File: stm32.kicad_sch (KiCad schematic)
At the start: 4 parts, among them U103 STM32G071KBTx

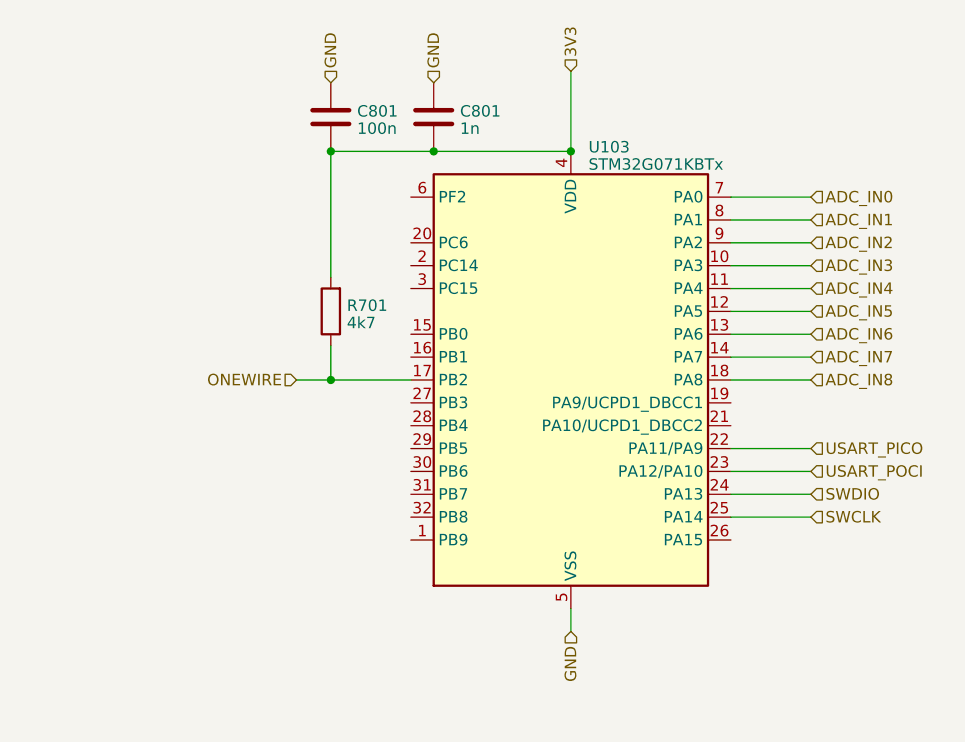
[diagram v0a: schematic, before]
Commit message: githubstart
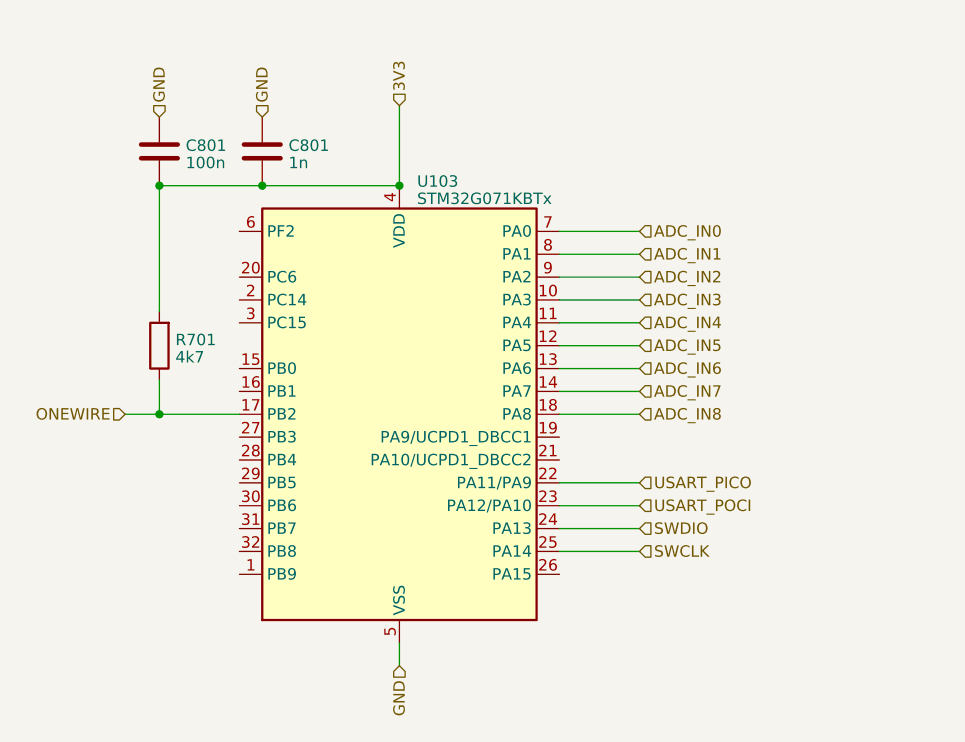
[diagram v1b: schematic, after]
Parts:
- removed C801: 1n, Capacitor_SMD:C_0603_1608Metric_Pad1.08x0.95mm_HandSolder, symbol Device:C
- removed C801: 100n, Capacitor_SMD:C_0603_1608Metric_Pad1.08x0.95mm_HandSolder, symbol Device:C
- added C801: 1n, Capacitor_SMD:C_0603_1608Metric_Pad1.08x0.95mm_HandSolder, symbol Device:C
- added C801: 100n, Capacitor_SMD:C_0603_1608Metric_Pad1.08x0.95mm_HandSolder, symbol Device:C
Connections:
- net 3V3: now also C801.1, C801.1
- net GND: now also C801.2, C801.2
